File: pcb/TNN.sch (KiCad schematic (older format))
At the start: 6 parts, among them P1 CONN_01X10, P2 CONN_01X04, P3 CONN_01X10, P4 CONN_01X04, SW1 SPST

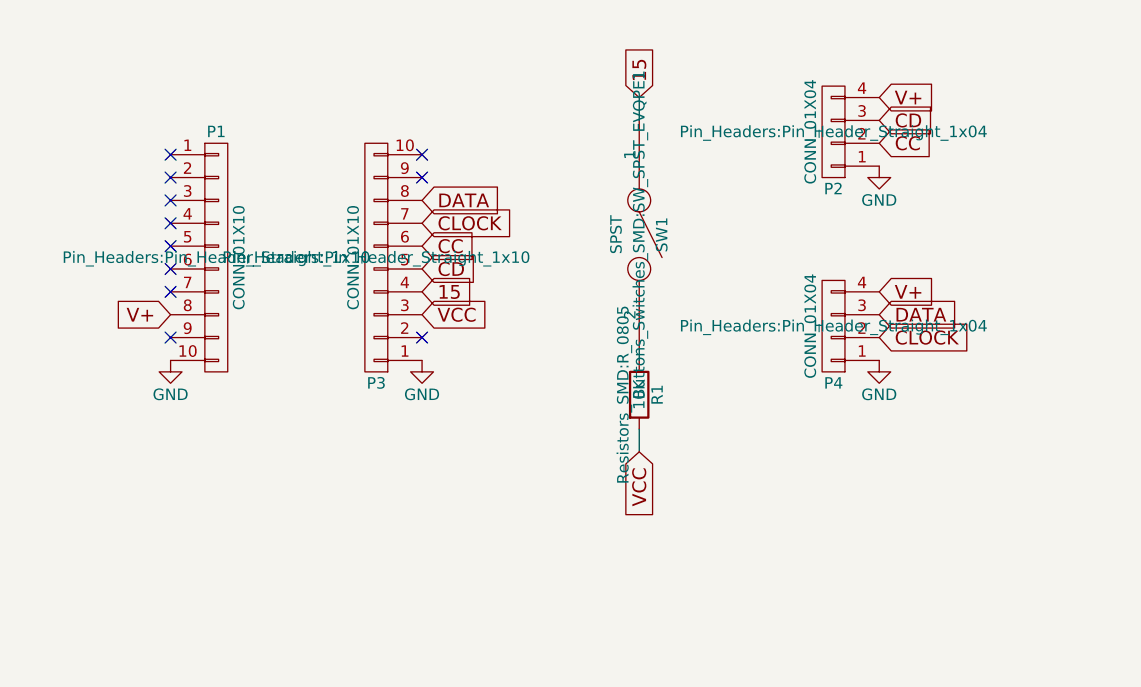
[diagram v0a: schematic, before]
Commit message: [*] Flip over.
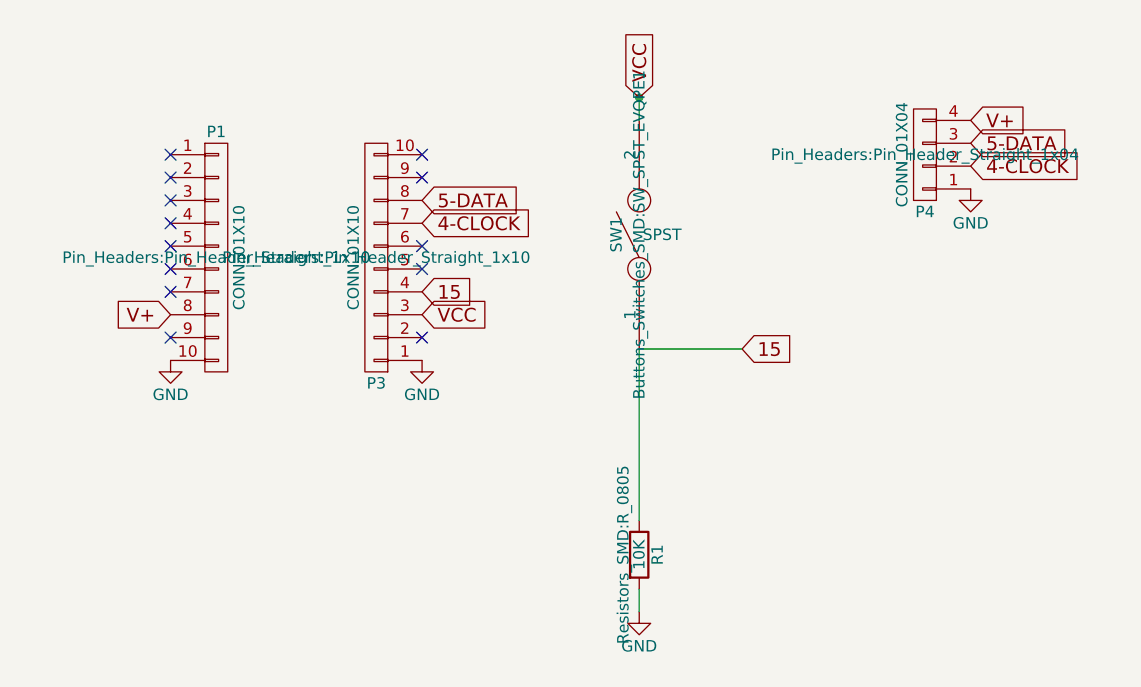
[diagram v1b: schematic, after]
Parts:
- removed P2: CONN_01X04, Pin_Headers:Pin_Header_Straight_1x04, symbol CONN_01X04
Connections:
- net 15: now also R1.1
- net GND: now also R1.2
- net VCC: now also SW1.2; no longer R1.2
- net CC: no longer names the net of P3.6 (P6)
- net CD: no longer names the net of P3.5 (P5)
- net CLOCK renamed 4-CLOCK
- net DATA renamed 5-DATA
- no-connect marks 11 -> 13
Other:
- moved on the sheet: P4, R1, SW1
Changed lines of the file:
@@
 $EndComp
 Text GLabel 2250 1300 2    60   Input ~ 0
-CLOCK
+4-CLOCK
 Text GLabel 2250 1200 2    60   Input ~ 0
-DATA
+5-DATA
 $Comp
 L R R1
 U 1 1 5808FF31
-P 3200 2050
-F 0 "R1" V 3280 2050 50  0000 C CNN
-F 1 "10K" V 3200 2050 50  0000 C CNN
-F 2 "Resistors_SMD:R_0805" V 3130 2050 50  0000 C CNN
-F 3 "" H 3200 2050 50  0000 C CNN
-	1    3200 2050
+P 3200 2750
+F 0 "R1" V 3280 2750 50  0000 C CNN
+F 1 "10K" V 3200 2750 50  0000 C CNN
+F 2 "Resistors_SMD:R_0805" V 3130 2750 50  0000 C CNN
+F 3 "" H 3200 2750 50  0000 C CNN
+	1    3200 2750
 	1    0    0    -1
 $EndComp
 Text GLabel 2250 1700 2    60   Input ~ 0
 VCC
-Text GLabel 3200 750  1    60   Input ~ 0
+Text GLabel 3650 1850 2    60   Input ~ 0
 15
 $Comp
 L GND #PWR01
-U 1 1 5808FBE5
-P 2250 1900
-F 0 "#PWR01" H 2250 1650 50  0001 C CNN
-F 1 "GND" H 2250 1750 50  0000 C CNN
-F 2 "" H 2250 1900 50  0000 C CNN
-F 3 "" H 2250 1900 50  0000 C CNN
-	1    2250 1900
-	1    0    0    -1
-$EndComp
-$Comp
-L GND #PWR02
 U 1 1 5808FC4B
 P 1150 1900
-F 0 "#PWR02" H 1150 1650 50  0001 C CNN
+F 0 "#PWR01" H 1150 1650 50  0001 C CNN
 F 1 "GND" H 1150 1750 50  0000 C CNN
 F 2 "" H 1150 1900 50  0000 C CNN
@@
 Text GLabel 2250 1600 2    60   Input ~ 0
 15
-Text GLabel 3200 2300 3    60   Input ~ 0
+Text GLabel 3200 750  1    60   Input ~ 0
 VCC
 $Comp
 L CONN_01X04 P4
 U 1 1 580905C2
-P 4050 1750
-F 0 "P4" H 4050 2000 50  0000 C CNN
-F 1 "CONN_01X04" V 4150 1750 50  0000 C CNN
-F 2 "Pin_Headers:Pin_Header_Straight_1x04" H 4050 1750 50  0000 C CNN
-F 3 "" H 4050 1750 50  0000 C CNN
-	1    4050 1750
+P 4450 1000
+F 0 "P4" H 4450 1250 50  0000 C CNN
+F 1 "CONN_01X04" V 4550 1000 50  0000 C CNN
+F 2 "Pin_Headers:Pin_Header_Straight_1x04" H 4450 1000 50  0000 C CNN
+F 3 "" H 4450 1000 50  0000 C CNN
+	1    4450 1000
 	-1   0    0    1
 $EndComp
 $Comp
-L GND #PWR05
+L GND #PWR02
 U 1 1 58090796
-P 4250 1900
-F 0 "#PWR05" H 4250 1650 50  0001 C CNN
-F 1 "GND" H 4250 1750 50  0000 C CNN
-F 2 "" H 4250 1900 50  0000 C CNN
-F 3 "" H 4250 1900 50  0000 C CNN
-	1    4250 1900
+P 4650 1150
+F 0 "#PWR02" H 4650 900 50  0001 C CNN
+F 1 "GND" H 4650 1000 50  0000 C CNN
+F 2 "" H 4650 1150 50  0000 C CNN
+F 3 "" H 4650 1150 50  0000 C CNN
+	1    4650 1150
 	1    0    0    -1
 $EndComp
-Text GLabel 4250 1700 2    60   Input ~ 0
-DATA
-Text GLabel 4250 1800 2    60   Input ~ 0
-CLOCK
-$Comp
-L CONN_01X04 P2
-U 1 1 580908DE
-P 4050 900
-F 0 "P2" H 4050 1150 50  0000 C CNN
-F 1 "CONN_01X04" V 4150 900 50  0000 C CNN
-F 2 "Pin_Headers:Pin_Header_Straight_1x04" H 4050 900 50  0000 C CNN
-F 3 "" H 4050 900 50  0000 C CNN
-	1    4050 900
-	-1   0    0    1
-$EndComp
-Text GLabel 2250 1500 2    60   Input ~ 0
-CD
-Text GLabel 2250 1400 2    60   Input ~ 0
-CC
-Text GLabel 4250 950  2    60   Input ~ 0
-CC
-Text GLabel 4250 850  2    60   Input ~ 0
-CD
-$Comp
-L GND #PWR07
-U 1 1 58090B86
-P 4250 1050
-F 0 "#PWR07" H 4250 800 50  0001 C CNN
-F 1 "GND" H 4250 900 50  0000 C CNN
-F 2 "" H 4250 1050 50  0000 C CNN
-F 3 "" H 4250 1050 50  0000 C CNN
-	1    4250 1050
-	1    0    0    -1
-$EndComp
+Text GLabel 4650 950  2    60   Input ~ 0
+5-DATA
+Text GLabel 4650 1050 2    60   Input ~ 0
+4-CLOCK
 $Comp
 L SPST SW1
@@
 P 3200 1350
 F 0 "SW1" H 3200 1450 50  0000 C CNN
-F 1 "SPST" H 3200 1250 50  0000 C CNN
+F 1 "SPST" V 3200 1250 50  0000 C CNN
 F 2 "Buttons_Switches_SMD:SW_SPST_EVQPE1" H 3200 1350 50  0000 C CNN
 F 3 "" H 3200 1350 50  0000 C CNN
 	1    3200 1350
-	0    1    1    0
+	0    -1   -1   0
 $EndComp
-Wire Wire Line
-	3200 1900 3200 1850
 Wire Wire Line
 	3200 750  3200 850
@@
 NoConn ~ 2250 1800
 NoConn ~ 1150 1800
-NoConn ~ 1150 1600
-NoConn ~ 1150 1400
 NoConn ~ 1150 1300
 NoConn ~ 1150 1200
 NoConn ~ 1150 1100
 NoConn ~ 1150 1000
-NoConn ~ 1150 1500
 Wire Wire Line
-	3200 2200 3200 2300
-Text GLabel 4250 1600 2    60   Input ~ 0
-V+
-Text GLabel 4250 750  2    60   Input ~ 0
+	3200 2900 3200 3000
+Text GLabel 4650 850  2    60   Input ~ 0
 V+
 Text GLabel 1150 1700 0    60   Input ~ 0
 V+
+NoConn ~ 2250 1400
+NoConn ~ 2250 1500
+$Comp
+L GND #PWR03
+U 1 1 580A5F4D
+P 3200 3000
+F 0 "#PWR03" H 3200 2750 50  0001 C CNN
+F 1 "GND" H 3200 2850 50  0000 C CNN
+F 2 "" H 3200 3000 50  0000 C CNN
+F 3 "" H 3200 3000 50  0000 C CNN
+	1    3200 3000
+	1    0    0    -1
+$EndComp
+Connection ~ 3200 750
+NoConn ~ 1150 1500
+NoConn ~ 1150 1600
+NoConn ~ 1150 1400
+$Comp
+L GND #PWR04
+U 1 1 5808FBE5
+P 2250 1900
+F 0 "#PWR04" H 2250 1650 50  0001 C CNN
+F 1 "GND" H 2250 1750 50  0000 C CNN
+F 2 "" H 2250 1900 50  0000 C CNN
+F 3 "" H 2250 1900 50  0000 C CNN
+	1    2250 1900
+	1    0    0    -1
+$EndComp
+Wire Wire Line
+	3650 1850 3200 1850
+Wire Wire Line
+	3200 1850 3200 2600
 $EndSCHEMATC
